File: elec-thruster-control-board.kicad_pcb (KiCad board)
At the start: 2 copper layers, 70 x 69 mm, 50 parts, among them J1 gp0-pwm0A, J10 gp17-pwm0B, J11 Conn_01x06, J12 Conn_01x06, J13 Conn_01x07, J2 gp2-pwm1A, J3 gp4-pwm2A, J4 gp6-pwm3A, J5 gp8-pwm4A, J6 gp27-pwm5B, J7 gp26-pwm5A, J8 gp21-pwm2B, J9 gp19-pwm1B

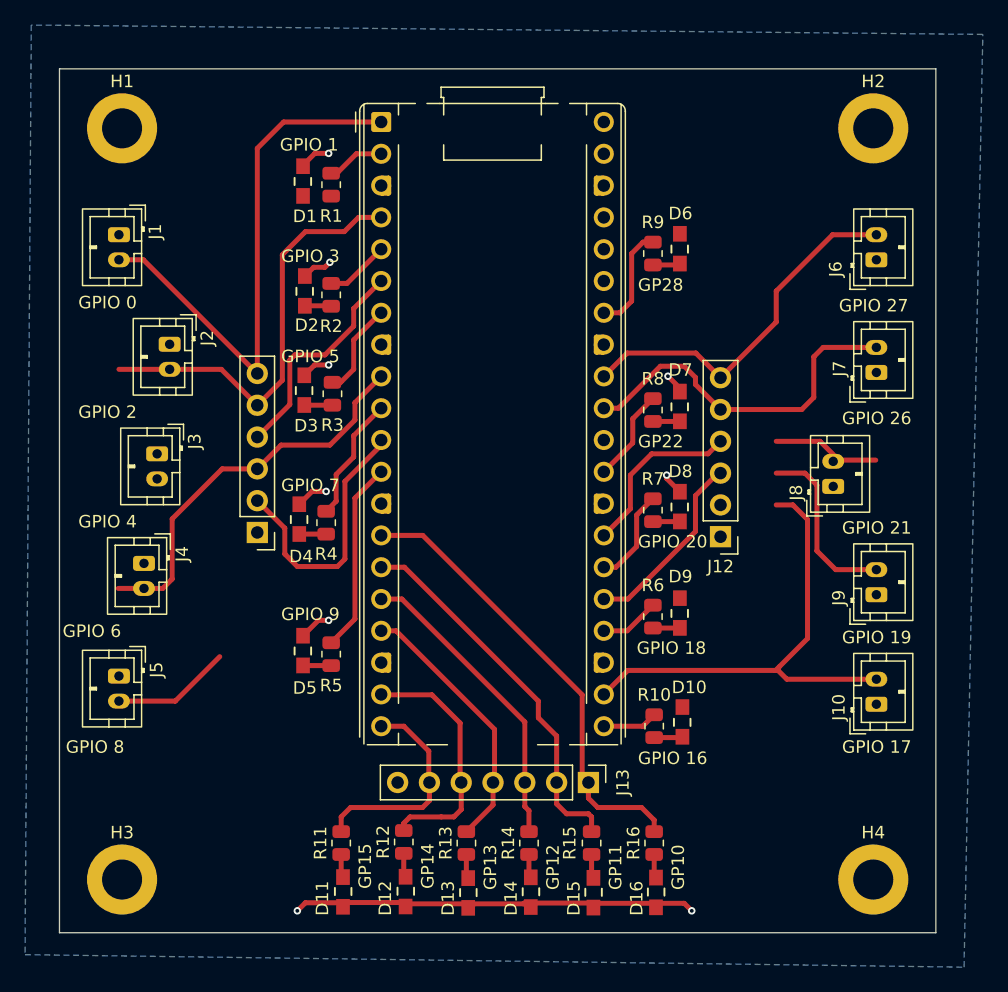
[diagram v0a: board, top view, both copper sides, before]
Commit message: Finished the job for Kekoa's compression
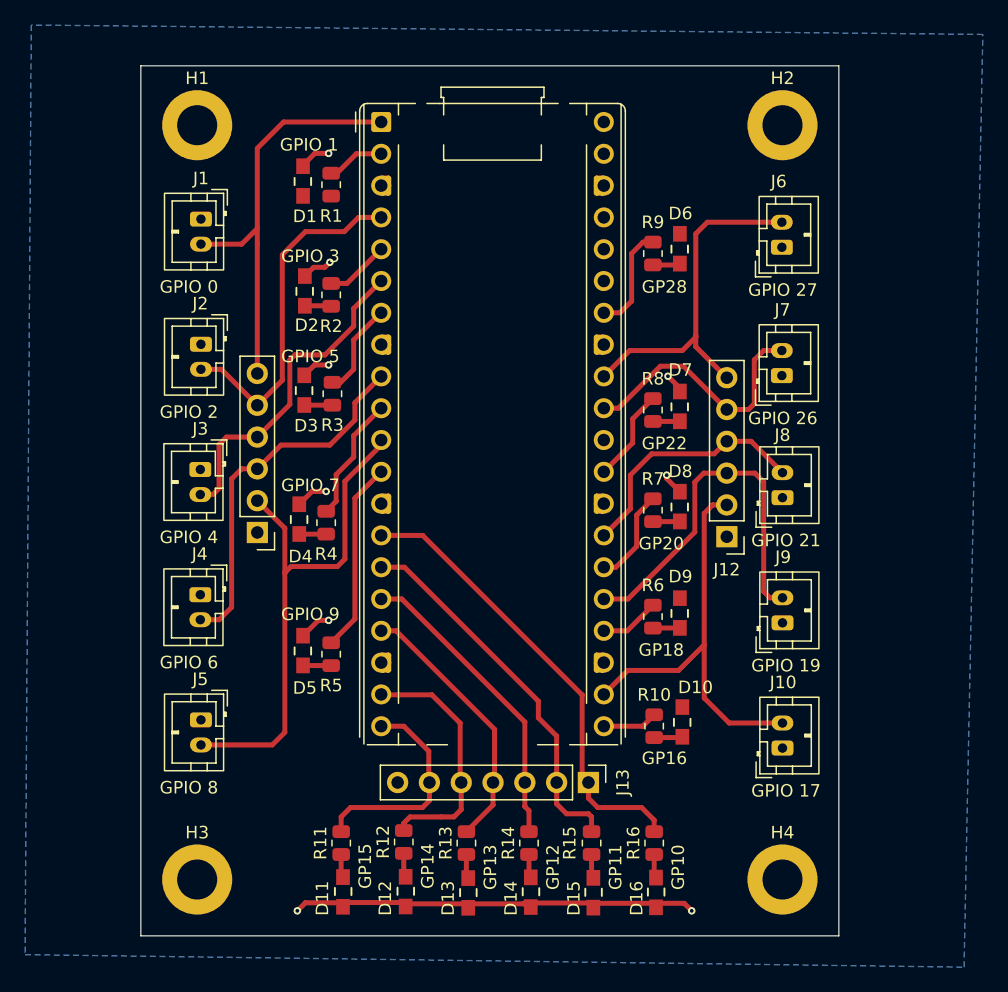
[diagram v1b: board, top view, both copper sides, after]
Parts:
- moved J10 8.28 mm to (162.8, 101.0)
- moved J9 7.83 mm to (162.8, 91.0)
- moved J6 7.62 mm to (162.7, 61.0)
- moved J7 7.55 mm to (162.7, 71.2)
- moved J5 7.43 mm to (116.3, 98.8)
- moved H2 7.25 mm to (162.8, 51.2)
- moved H4 7.25 mm to (162.8, 111.5)
- moved J1 6.67 mm to (116.3, 58.8)
- moved H1 6.01 mm to (116.0, 51.2)
- moved H3 6.00 mm to (116.0, 111.5)
- moved J4 5.15 mm to (116.2, 88.8)
- moved J8 4.15 mm to (162.8, 81.0)
- moved J3 3.67 mm to (116.2, 78.8)
- moved J2 2.50 mm to (116.3, 68.8)
- moved J12 0.50 mm to (158.3, 84.1)
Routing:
- net /gp8-pwm4A: track 30.9 -> 42.5 mm
- net /gp0-pwm0A: track 43.6 -> 34.1 mm
- net /gp4-pwm2A: track 18.0 -> 26.5 mm
- net /gp26-pwm5A: track 28.9 -> 21.0 mm
- net /gp2-pwm1A: track 34.2 -> 27.7 mm
- net /gp17-pwm0B: track 38.9 -> 33.6 mm
- net /gp21-pwm2B: track 22.6 -> 20.0 mm
- net /gp6-pwm3A: track 32.1 -> 29.8 mm
- net /gp27-pwm5B: track 29.5 -> 28.6 mm
- net /gp19-pwm1B: track 29.5 -> 30.0 mm
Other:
- board size 70 x 69 mm -> 55.8 x 69.5 mm
- board text added: "GP16"
- board text added: "GP18"
- board text added: "GP20"
- board text removed: "GPIO 16"
- board text removed: "GPIO 18"
- board text removed: "GPIO 20"
